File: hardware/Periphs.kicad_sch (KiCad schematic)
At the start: 12 parts, among them J6 Conn_01x04, U1 TCAN4551RGYRQ1, Y3 SG-8002LB

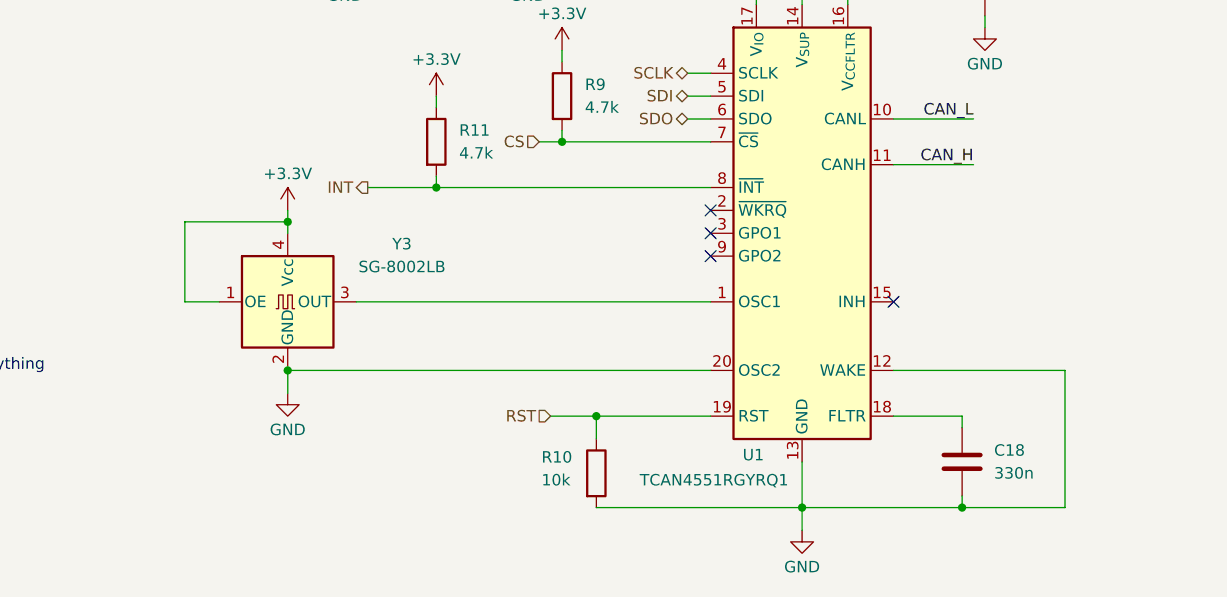
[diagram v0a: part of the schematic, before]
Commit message: some changes`
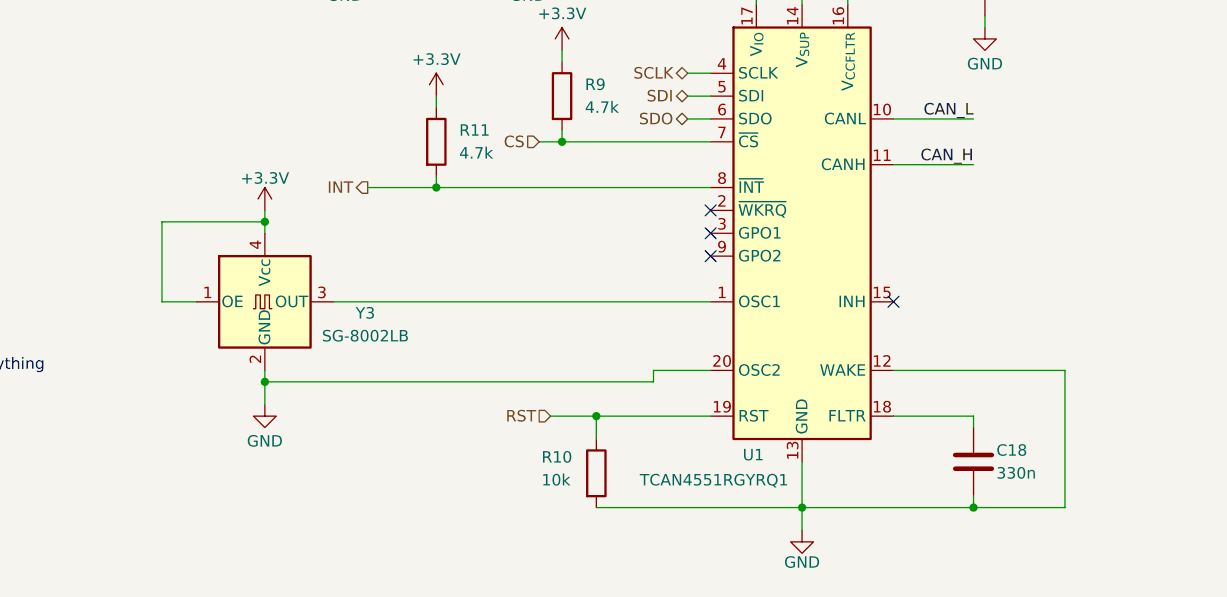
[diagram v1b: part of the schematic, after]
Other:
- moved on the sheet: C18, Y3
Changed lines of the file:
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@@
 	)
 	(junction
-		(at 99.06 104.14)
+		(at 115.57 83.82)
 		(diameter 0)
 		(color 0 0 0 0)
 	)
 	(junction
-		(at 115.57 83.82)
+		(at 96.52 105.41)
 		(diameter 0)
 		(color 0 0 0 0)
@@
 	)
 	(junction
-		(at 173.99 119.38)
+		(at 96.52 87.63)
 		(diameter 0)
 		(color 0 0 0 0)
 	)
 	(junction
-		(at 99.06 87.63)
+		(at 105.41 46.99)
 		(diameter 0)
 		(color 0 0 0 0)
 	)
 	(junction
-		(at 105.41 46.99)
+		(at 175.26 119.38)
 		(diameter 0)
 		(color 0 0 0 0)
@@
 	(wire
 		(pts
-			(xy 173.99 109.22) (xy 173.99 110.49)
+			(xy 175.26 109.22) (xy 175.26 110.49)
 		)
 		(stroke
@@
 	(wire
 		(pts
-			(xy 99.06 86.36) (xy 99.06 87.63)
+			(xy 96.52 86.36) (xy 96.52 87.63)
 		)
 		(stroke
@@
 	(wire
 		(pts
-			(xy 166.37 109.22) (xy 173.99 109.22)
+			(xy 139.7 105.41) (xy 139.7 104.14)
 		)
 		(stroke
@@
 	(wire
 		(pts
-			(xy 125.73 57.15) (xy 135.89 57.15)
+			(xy 166.37 109.22) (xy 175.26 109.22)
 		)
 		(stroke
@@
 	(wire
 		(pts
-			(xy 105.41 44.45) (xy 105.41 46.99)
+			(xy 125.73 57.15) (xy 135.89 57.15)
 		)
 		(stroke
@@
 	(wire
 		(pts
-			(xy 156.21 119.38) (xy 173.99 119.38)
+			(xy 105.41 44.45) (xy 105.41 46.99)
 		)
 		(stroke
@@
 	(wire
 		(pts
-			(xy 105.41 46.99) (xy 115.57 46.99)
+			(xy 156.21 119.38) (xy 175.26 119.38)
 		)
 		(stroke
@@
 	(wire
 		(pts
-			(xy 220.98 83.82) (xy 227.33 83.82)
+			(xy 105.41 46.99) (xy 115.57 46.99)
 		)
 		(stroke
@@
 	(wire
 		(pts
-			(xy 173.99 118.11) (xy 173.99 119.38)
+			(xy 220.98 83.82) (xy 227.33 83.82)
 		)
 		(stroke
@@
 	(wire
 		(pts
-			(xy 185.42 119.38) (xy 173.99 119.38)
+			(xy 125.73 48.26) (xy 125.73 46.99)
 		)
 		(stroke
@@
 	(wire
 		(pts
-			(xy 99.06 104.14) (xy 146.05 104.14)
+			(xy 105.41 57.15) (xy 105.41 58.42)
 		)
 		(stroke
@@
 	(wire
 		(pts
-			(xy 125.73 48.26) (xy 125.73 46.99)
+			(xy 125.73 57.15) (xy 125.73 58.42)
 		)
 		(stroke
@@
 	(wire
 		(pts
-			(xy 105.41 57.15) (xy 105.41 58.42)
+			(xy 156.21 119.38) (xy 156.21 121.92)
 		)
 		(stroke
@@
 	(wire
 		(pts
-			(xy 125.73 57.15) (xy 125.73 58.42)
+			(xy 96.52 105.41) (xy 139.7 105.41)
 		)
 		(stroke
@@
 	(wire
 		(pts
-			(xy 156.21 119.38) (xy 156.21 121.92)
+			(xy 143.51 73.66) (xy 146.05 73.66)
 		)
 		(stroke
@@
 	(wire
 		(pts
-			(xy 143.51 73.66) (xy 146.05 73.66)
+			(xy 129.54 77.47) (xy 129.54 78.74)
 		)
 		(stroke
@@
 	(wire
 		(pts
-			(xy 129.54 77.47) (xy 129.54 78.74)
+			(xy 127 78.74) (xy 129.54 78.74)
 		)
 		(stroke
@@
 	(wire
 		(pts
-			(xy 127 78.74) (xy 129.54 78.74)
+			(xy 125.73 44.45) (xy 125.73 46.99)
 		)
 		(stroke
@@
 	(wire
 		(pts
-			(xy 125.73 44.45) (xy 125.73 46.99)
+			(xy 125.73 46.99) (xy 135.89 46.99)
 		)
 		(stroke
@@
 	(wire
 		(pts
-			(xy 125.73 46.99) (xy 135.89 46.99)
+			(xy 85.09 87.63) (xy 96.52 87.63)
 		)
 		(stroke
@@
 	(wire
 		(pts
-			(xy 87.63 87.63) (xy 99.06 87.63)
+			(xy 156.21 55.88) (xy 156.21 63.5)
 		)
 		(stroke
@@
 	(wire
 		(pts
-			(xy 156.21 55.88) (xy 156.21 63.5)
+			(xy 175.26 118.11) (xy 175.26 119.38)
 		)
 		(stroke
@@
 	(wire
 		(pts
-			(xy 91.44 96.52) (xy 87.63 96.52)
+			(xy 88.9 96.52) (xy 85.09 96.52)
 		)
 		(stroke
@@
 	(wire
 		(pts
-			(xy 87.63 96.52) (xy 87.63 87.63)
+			(xy 85.09 96.52) (xy 85.09 87.63)
 		)
 		(stroke
@@
 	(wire
 		(pts
-			(xy 133.35 109.22) (xy 146.05 109.22)
+			(xy 139.7 104.14) (xy 146.05 104.14)
 		)
 		(stroke
@@
 	(wire
 		(pts
-			(xy 99.06 104.14) (xy 99.06 106.68)
+			(xy 96.52 105.41) (xy 96.52 104.14)
+		)
+		(stroke
+			(width 0)
+			(type default)
+		)
+	)
+	(wire
+		(pts
+			(xy 133.35 109.22) (xy 146.05 109.22)
 		)
 		(stroke
@@
 	(wire
 		(pts
-			(xy 106.68 96.52) (xy 146.05 96.52)
+			(xy 104.14 96.52) (xy 146.05 96.52)
 		)
 		(stroke
@@
 	(wire
 		(pts
+			(xy 175.26 119.38) (xy 185.42 119.38)
+		)
+		(stroke
+			(width 0)
+			(type default)
+		)
+	)
+	(wire
+		(pts
 			(xy 220.98 76.2) (xy 227.33 76.2)
 		)
@@
 	(wire
 		(pts
-			(xy 99.06 87.63) (xy 99.06 88.9)
+			(xy 96.52 105.41) (xy 96.52 107.95)
+		)
+		(stroke
+			(width 0)
+			(type default)
+		)
+	)
+	(wire
+		(pts
+			(xy 96.52 87.63) (xy 96.52 88.9)
 		)
 		(stroke
@@
 	)
 	(image
-		(at 157.48 129.54)
+		(at 157.48 132.08)
 		(scale 0.238773)
 		(data "iVBORw0KGgoAAAANSUhEUgAABqIAAACCCAYAAAAt69luAAAMTWlDQ1BJQ0MgUHJvZmlsZQAASImV"
@@
 		)
 		(property "Value" "GND"
-			(at 156.21 125.984 0)
+			(at 156.21 125.476 0)
 			(show_name no)
 			(do_not_autoplace no)
@@
 	(symbol
 		(lib_id "power:+3.3V")
-		(at 99.06 86.36 0)
+		(at 96.52 86.36 0)
 		(unit 1)
 		(body_style 1)
@@
 		(dnp no)
 		(property "Reference" "#PWR039"
-			(at 99.06 90.17 0)
+			(at 96.52 90.17 0)
 			(hide yes)
 			(show_name no)
@@
 		)
 		(property "Value" "+3.3V"
-			(at 99.06 82.296 0)
+			(at 96.52 82.804 0)
 			(show_name no)
 			(do_not_autoplace no)
@@
 		)
 		(property "Footprint" ""
-			(at 99.06 86.36 0)
+			(at 96.52 86.36 0)
 			(hide yes)
 			(show_name no)
@@
 		)
 		(property "Datasheet" ""
-			(at 99.06 86.36 0)
+			(at 96.52 86.36 0)
 			(hide yes)
 			(show_name no)
@@
 		)
 		(property "Description" "Power symbol creates a global label with name \"+3.3V\""
-			(at 99.06 86.36 0)
+			(at 96.52 86.36 0)
 			(hide yes)
 			(show_name no)
@@
 	(symbol
 		(lib_id "Oscillator:SG-8002LB")
-		(at 99.06 96.52 0)
+		(at 96.52 96.52 0)
 		(unit 1)
 		(body_style 1)
@@
 		(in_pos_files yes)
 		(dnp no)
-		(fields_autoplaced yes)
 		(property "Reference" "Y3"
-			(at 111.76 90.0998 0)
+			(at 107.696 97.79 0)
 			(show_name no)
 			(do_not_autoplace no)
@@
 		)
 		(property "Value" "SG-8002LB"
-			(at 111.76 92.6398 0)
+			(at 107.696 100.33 0)
 			(show_name no)
 			(do_not_autoplace no)
@@
 		)
 		(property "Footprint" "Oscillator:Oscillator_SMD_SeikoEpson_SG8002LB-4Pin_5.0x3.2mm"
-			(at 116.84 105.41 0)
+			(at 114.3 105.41 0)
 			(hide yes)
 			(show_name no)
@@
 		)
 		(property "Datasheet" "https://support.epson.biz/td/api/doc_check.php?dl=brief_SG-8002LB&lang=en"
-			(at 96.52 96.52 0)
+			(at 93.98 96.52 0)
 			(hide yes)
 			(show_name no)
@@
 		)
 		(property "Description" "CMOS Clock Oscillator 1 to 125 MHz"
-			(at 99.06 96.52 0)
+			(at 96.52 96.52 0)
 			(hide yes)
 			(show_name no)
@@
 	(symbol
 		(lib_id "Device:C")
-		(at 173.99 114.3 0)
+		(at 175.26 114.3 0)
 		(unit 1)
 		(body_style 1)
@@
 		(dnp no)
 		(property "Reference" "C18"
-			(at 177.546 113.03 0)
+			(at 177.8 113.03 0)
 			(show_name no)
 			(do_not_autoplace no)
@@
 		)
 		(property "Value" "330n"
-			(at 177.546 115.57 0)
+			(at 177.8 115.57 0)
 			(show_name no)
 			(do_not_autoplace no)
@@
 		)
 		(property "Footprint" ""
-			(at 174.9552 118.11 0)
+			(at 176.2252 118.11 0)
 			(hide yes)
 			(show_name no)
@@
 		)
 		(property "Datasheet" ""
-			(at 173.99 114.3 0)
+			(at 175.26 114.3 0)
 			(hide yes)
 			(show_name no)
@@
 		)
 		(property "Description" "Unpolarized capacitor"
-			(at 173.99 114.3 0)
+			(at 175.26 114.3 0)
 			(hide yes)
 			(show_name no)
@@
 	(symbol
 		(lib_id "power:GND")
-		(at 99.06 106.68 0)
+		(at 96.52 107.95 0)
 		(unit 1)
 		(body_style 1)
@@
 		(dnp no)
 		(property "Reference" "#PWR040"
-			(at 99.06 113.03 0)
+			(at 96.52 114.3 0)
 			(hide yes)
 			(show_name no)
@@
 		)
 		(property "Value" "GND"
-			(at 99.06 110.744 0)
+			(at 96.52 112.014 0)
 			(show_name no)
 			(do_not_autoplace no)
@@
 		)
 		(property "Footprint" ""
-			(at 99.06 106.68 0)
+			(at 96.52 107.95 0)
 			(hide yes)
 			(show_name no)
@@
 		)
 		(property "Datasheet" ""
-			(at 99.06 106.68 0)
+			(at 96.52 107.95 0)
 			(hide yes)
 			(show_name no)
@@
 		)
 		(property "Description" "Power symbol creates a global label with name \"GND\" , ground"
-			(at 99.06 106.68 0)
+			(at 96.52 107.95 0)
 			(hide yes)
 			(show_name no)
